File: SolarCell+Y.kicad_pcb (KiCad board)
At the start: 6 copper layers, 50 x 50 mm, 27 parts, among them IC1 symbols_TSL2561, Q1 IRLML2803

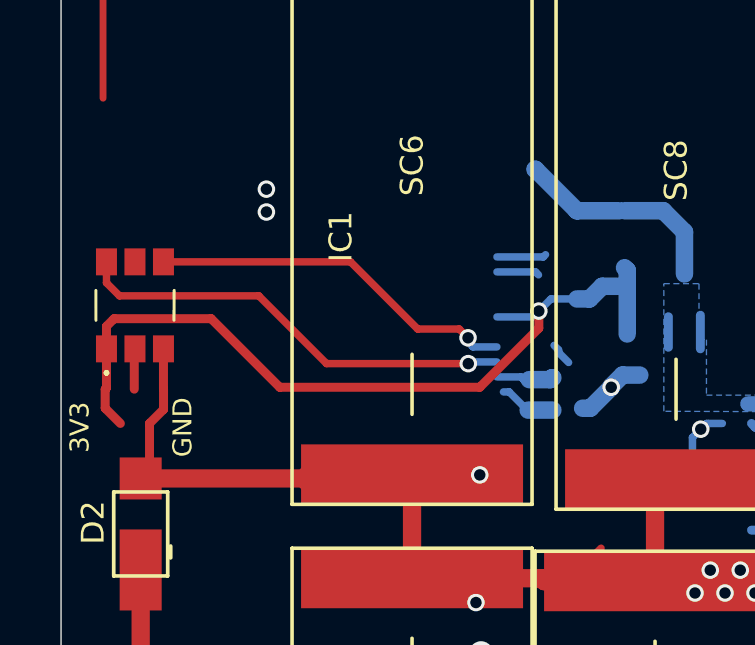
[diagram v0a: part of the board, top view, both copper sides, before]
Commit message: Massaged J1 into there somehow.
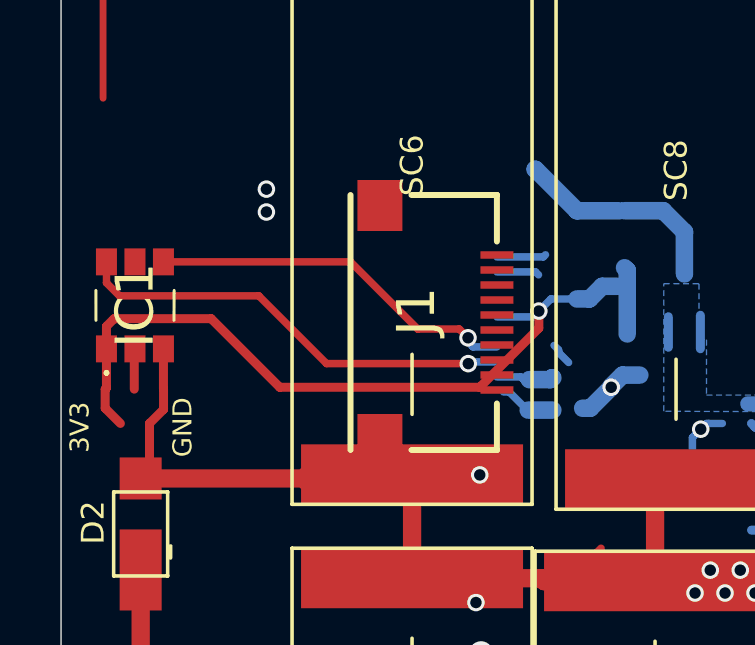
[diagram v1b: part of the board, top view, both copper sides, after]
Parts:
- added J1: symbols_XF2M-1015-1A, solarpcb:XF2M-1015-1A, F.Cu at (164.5, 58.0)
- IC1: footprint custom-footprints:TSL2561 -> solarpcb:TSL2561
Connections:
- IC1 pad 1: (no net) -> +3V3
- IC1 pad 2: (no net) -> Net-(IC1-Pad2)
- IC1 pad 3: (no net) -> GND
- IC1 pad 4: (no net) -> SCL1
- IC1 pad 6: (no net) -> SDA1
- R1 pad 1: (no net) -> +3V3
- R4 pad 1: (no net) -> BATT_N
- R7 pad 2: (no net) -> BATT_P
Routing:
- net (no net): track 83.2 -> 41.1 mm, vias 7 -> 4
- net +3V3: track 2.24 -> 27.0 mm, vias 0 -> 1
- net SDA1: track 0.00 -> 14.9 mm, vias 0 -> 1
- net SCL1: track 0.00 -> 12.4 mm, vias 0 -> 1
- net Net-(H1-Pad1): track 11.2 -> 0.00 mm
- net Net-(IC1-Pad2): track 3.87 -> 5.22 mm
